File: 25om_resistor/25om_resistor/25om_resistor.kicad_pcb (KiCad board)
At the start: 2 copper layers, 24.2 x 21.9 mm, 11 parts, among them J1 Conn_01x02_Female

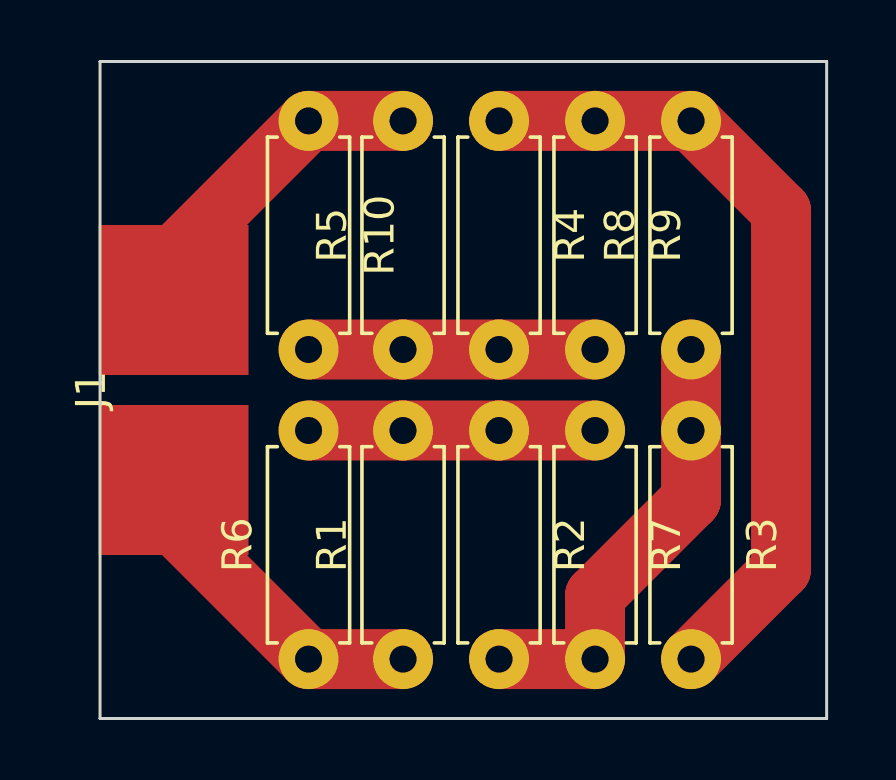
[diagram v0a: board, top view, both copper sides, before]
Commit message: Cleanup
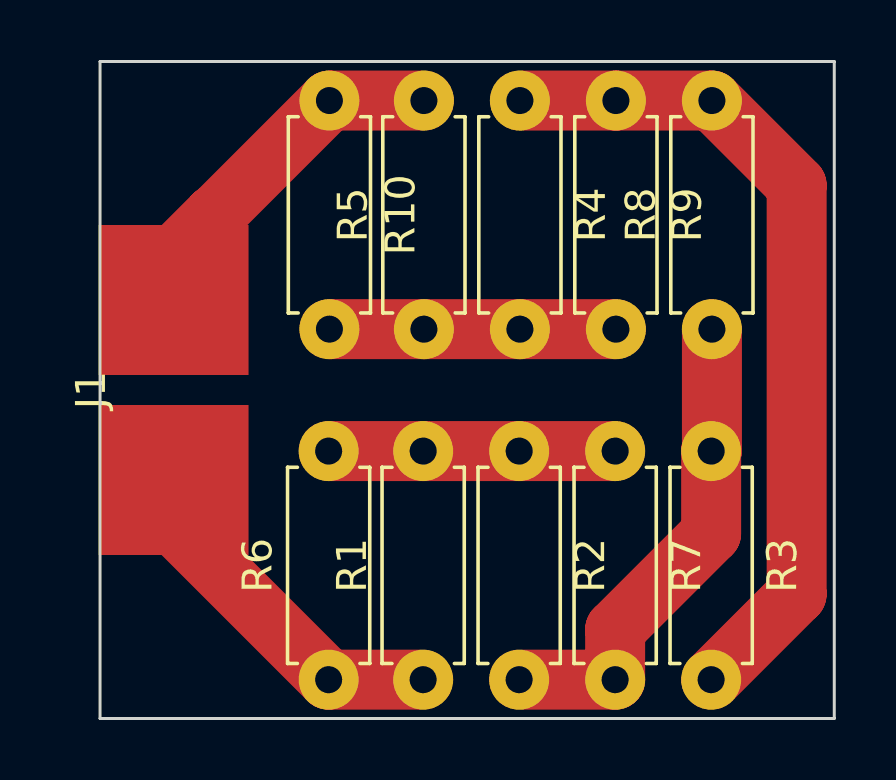
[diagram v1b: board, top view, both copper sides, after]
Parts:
- moved R4 0.97 mm to (64.8, 28.7)
- moved R9 0.97 mm to (68.0, 28.7)
- moved R10 0.97 mm to (58.4, 28.7)
- moved R5 0.97 mm to (61.6, 36.3)
- moved R8 0.97 mm to (71.2, 36.3)
- moved R1 0.96 mm to (61.6, 48.0)
- moved R2 0.96 mm to (64.8, 40.4)
- moved R3 0.96 mm to (71.2, 40.4)
- moved R6 0.96 mm to (58.4, 48.0)
- moved R7 0.96 mm to (68.0, 40.4)
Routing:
- net Net-(R2-Pad2): track 14.8 -> 16.2 mm
- net Net-(R3-Pad2): track 26.8 -> 28.1 mm
- net Net-(J1-Pad2): track 11.0 -> 12.0 mm
- net Net-(J1-Pad1): track 11.0 -> 11.9 mm
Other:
- board size 24.2 x 21.9 mm -> 24.5 x 21.9 mm
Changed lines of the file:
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@@
     (pad_to_mask_clearance 0)
     (pcbplotparams
-      (layerselection 0x00010fc_ffffffff)
+      (layerselection 0x0001000_7fffffff)
       (disableapertmacros false)
       (usegerberextensions false)
@@
       (outputformat 1)
       (mirror false)
-      (drillshape 1)
+      (drillshape 0)
       (scaleselection 1)
-      (outputdirectory "")
+      (outputdirectory "out/")
     )
   )
@@
   (net 6 "Net-(R10-Pad2)")
   (footprint "Resistor_THT:R_Axial_DIN0207_L6.3mm_D2.5mm_P7.62mm_Horizontal" (layer "F.Cu")
-    (at 67.3 39.7 -90)
+    (at 67.97 40.386 -90)
     (descr "Resistor, Axial_DIN0207 series, Axial, Horizontal, pin pitch=7.62mm, 0.25W = 1/4W, length*diameter=6.3*2.5mm^2, http://cdn-reichelt.de/documents/datenblatt/B400/1_4W%23YAG.pdf")
     (tags "Resistor Axial_DIN0207 series Axial Horizontal pin pitch 7.62mm 0.25W = 1/4W length 6.3mm diameter 2.5mm")
@@
   )
   (footprint "Resistor_THT:R_Axial_DIN0207_L6.3mm_D2.5mm_P7.62mm_Horizontal" (layer "F.Cu")
-    (at 57.75 47.32 90)
+    (at 58.42 48.006 90)
     (descr "Resistor, Axial_DIN0207 series, Axial, Horizontal, pin pitch=7.62mm, 0.25W = 1/4W, length*diameter=6.3*2.5mm^2, http://cdn-reichelt.de/documents/datenblatt/B400/1_4W%23YAG.pdf")
     (tags "Resistor Axial_DIN0207 series Axial Horizontal pin pitch 7.62mm 0.25W = 1/4W length 6.3mm diameter 2.5mm")
@@
   )
   (footprint "Resistor_THT:R_Axial_DIN0207_L6.3mm_D2.5mm_P7.62mm_Horizontal" (layer "F.Cu")
-    (at 70.5 37 90)
+    (at 71.195 36.322 90)
     (descr "Resistor, Axial_DIN0207 series, Axial, Horizontal, pin pitch=7.62mm, 0.25W = 1/4W, length*diameter=6.3*2.5mm^2, http://cdn-reichelt.de/documents/datenblatt/B400/1_4W%23YAG.pdf")
     (tags "Resistor Axial_DIN0207 series Axial Horizontal pin pitch 7.62mm 0.25W = 1/4W length 6.3mm diameter 2.5mm")
@@
   )
   (footprint "Resistor_THT:R_Axial_DIN0207_L6.3mm_D2.5mm_P7.62mm_Horizontal" (layer "F.Cu")
-    (at 60.9 37 90)
+    (at 61.595 36.322 90)
     (descr "Resistor, Axial_DIN0207 series, Axial, Horizontal, pin pitch=7.62mm, 0.25W = 1/4W, length*diameter=6.3*2.5mm^2, http://cdn-reichelt.de/documents/datenblatt/B400/1_4W%23YAG.pdf")
     (tags "Resistor Axial_DIN0207 series Axial Horizontal pin pitch 7.62mm 0.25W = 1/4W length 6.3mm diameter 2.5mm")
@@
   )
   (footprint "Resistor_THT:R_Axial_DIN0207_L6.3mm_D2.5mm_P7.62mm_Horizontal" (layer "F.Cu")
-    (at 64.1 29.38 -90)
+    (at 64.795 28.702 -90)
     (descr "Resistor, Axial_DIN0207 series, Axial, Horizontal, pin pitch=7.62mm, 0.25W = 1/4W, length*diameter=6.3*2.5mm^2, http://cdn-reichelt.de/documents/datenblatt/B400/1_4W%23YAG.pdf")
     (tags "Resistor Axial_DIN0207 series Axial Horizontal pin pitch 7.62mm 0.25W = 1/4W length 6.3mm diameter 2.5mm")
@@
   )
   (footprint "Resistor_THT:R_Axial_DIN0207_L6.3mm_D2.5mm_P7.62mm_Horizontal" (layer "F.Cu")
-    (at 70.5 39.7 -90)
+    (at 71.17 40.386 -90)
     (descr "Resistor, Axial_DIN0207 series, Axial, Horizontal, pin pitch=7.62mm, 0.25W = 1/4W, length*diameter=6.3*2.5mm^2, http://cdn-reichelt.de/documents/datenblatt/B400/1_4W%23YAG.pdf")
     (tags "Resistor Axial_DIN0207 series Axial Horizontal pin pitch 7.62mm 0.25W = 1/4W length 6.3mm diameter 2.5mm")
@@
   )
   (footprint "Resistor_THT:R_Axial_DIN0207_L6.3mm_D2.5mm_P7.62mm_Horizontal" (layer "F.Cu")
-    (at 57.75 29.38 -90)
+    (at 58.445 28.702 -90)
     (descr "Resistor, Axial_DIN0207 series, Axial, Horizontal, pin pitch=7.62mm, 0.25W = 1/4W, length*diameter=6.3*2.5mm^2, http://cdn-reichelt.de/documents/datenblatt/B400/1_4W%23YAG.pdf")
     (tags "Resistor Axial_DIN0207 series Axial Horizontal pin pitch 7.62mm 0.25W = 1/4W length 6.3mm diameter 2.5mm")
@@
   )
   (footprint "Resistor_THT:R_Axial_DIN0207_L6.3mm_D2.5mm_P7.62mm_Horizontal" (layer "F.Cu")
-    (at 60.9 47.32 90)
+    (at 61.57 48.006 90)
     (descr "Resistor, Axial_DIN0207 series, Axial, Horizontal, pin pitch=7.62mm, 0.25W = 1/4W, length*diameter=6.3*2.5mm^2, http://cdn-reichelt.de/documents/datenblatt/B400/1_4W%23YAG.pdf")
     (tags "Resistor Axial_DIN0207 series Axial Horizontal pin pitch 7.62mm 0.25W = 1/4W length 6.3mm diameter 2.5mm")
@@
   )
   (footprint "Resistor_THT:R_Axial_DIN0207_L6.3mm_D2.5mm_P7.62mm_Horizontal" (layer "F.Cu")
-    (at 64.1 39.7 -90)
+    (at 64.77 40.386 -90)
     (descr "Resistor, Axial_DIN0207 series, Axial, Horizontal, pin pitch=7.62mm, 0.25W = 1/4W, length*diameter=6.3*2.5mm^2, http://cdn-reichelt.de/documents/datenblatt/B400/1_4W%23YAG.pdf")
     (tags "Resistor Axial_DIN0207 series Axial Horizontal pin pitch 7.62mm 0.25W = 1/4W length 6.3mm diameter 2.5mm")
@@
       (effects (font (size 1 1) (thickness 0.15)))
     )
-    (fp_text value "Conn_01x02_Female" (at 3 2.75 90) (layer "F.Fab")
+    (fp_text value "Conn_01x02_Female" (at 2.992 4.115 90) (layer "F.Fab")
       (effects (font (size 1 1) (thickness 0.15)))
     )
@@
   )
   (footprint "Resistor_THT:R_Axial_DIN0207_L6.3mm_D2.5mm_P7.62mm_Horizontal" (layer "F.Cu")
-    (at 67.3 29.38 -90)
+    (at 67.995 28.702 -90)
     (descr "Resistor, Axial_DIN0207 series, Axial, Horizontal, pin pitch=7.62mm, 0.25W = 1/4W, length*diameter=6.3*2.5mm^2, http://cdn-reichelt.de/documents/datenblatt/B400/1_4W%23YAG.pdf")
     (tags "Resistor Axial_DIN0207 series Axial Horizontal pin pitch 7.62mm 0.25W = 1/4W length 6.3mm diameter 2.5mm")
@@
     )
   )
-  (gr_rect (start 50.8 27.4) (end 75.02 49.3) (layer "Edge.Cuts") (width 0.1) (fill none))
-  (segment (start 57.75 47.32) (end 60.9 47.32) (width 2) (layer "F.Cu") (net 1))
-  (segment (start 53.25 42.82) (end 57.75 47.32) (width 2) (layer "F.Cu") (net 1))
-  (segment (start 53.25 41.35) (end 53.25 42.82) (width 2) (layer "F.Cu") (net 1))
-  (segment (start 53.25 33.88) (end 57.75 29.38) (width 2) (layer "F.Cu") (net 2))
-  (segment (start 53.25 35.35) (end 53.25 33.88) (width 2) (layer "F.Cu") (net 2))
-  (segment (start 57.75 29.38) (end 60.9 29.38) (width 2) (layer "F.Cu") (net 2))
-  (segment (start 57.75 39.7) (end 60.9 39.7) (width 2) (layer "F.Cu") (net 3))
-  (segment (start 60.9 39.7) (end 64.1 39.7) (width 2) (layer "F.Cu") (net 3))
-  (segment (start 64.1 39.7) (end 67.3 39.7) (width 2) (layer "F.Cu") (net 3))
-  (segment (start 64.1 47.32) (end 67.3 47.32) (width 2) (layer "F.Cu") (net 4))
-  (segment (start 67.3 47.32) (end 67.3 45.2) (width 2) (layer "F.Cu") (net 4))
-  (segment (start 67.3 45.2) (end 70.5 42) (width 2) (layer "F.Cu") (net 4))
-  (segment (start 70.5 42) (end 70.5 39.7) (width 2) (layer "F.Cu") (net 4))
-  (segment (start 70.5 39.7) (end 70.5 37) (width 2) (layer "F.Cu") (net 4))
-  (segment (start 73.5 32.38) (end 73.5 44.32) (width 2) (layer "F.Cu") (net 5))
-  (segment (start 73.5 44.32) (end 70.5 47.32) (width 2) (layer "F.Cu") (net 5))
-  (segment (start 67.3 29.38) (end 70.5 29.38) (width 2) (layer "F.Cu") (net 5))
-  (segment (start 64.1 29.38) (end 67.3 29.38) (width 2) (layer "F.Cu") (net 5))
-  (segment (start 70.5 29.38) (end 73.5 32.38) (width 2) (layer "F.Cu") (net 5))
-  (segment (start 64.1 37) (end 67.3 37) (width 2) (layer "F.Cu") (net 6))
-  (segment (start 64.1 37) (end 60.9 37) (width 2) (layer "F.Cu") (net 6))
-  (segment (start 57.75 37) (end 60.9 37) (width 2) (layer "F.Cu") (net 6))
+  (gr_rect (start 50.8 27.4) (end 75.274 49.3) (layer "Edge.Cuts") (width 0.1) (fill none))
+  (segment (start 58.42 48.006) (end 61.57 48.006) (width 2) (layer "F.Cu") (net 1))
+  (segment (start 53.25 41.35) (end 53.25 42.836) (width 2) (layer "F.Cu") (net 1))
+  (segment (start 53.25 42.836) (end 58.42 48.006) (width 2) (layer "F.Cu") (net 1))
+  (segment (start 54.635 32.512) (end 54.61 32.512) (width 2) (layer "F.Cu") (net 2))
+  (segment (start 54.61 32.512) (end 53.25 33.872) (width 2) (layer "F.Cu") (net 2))
+  (segment (start 53.25 33.872) (end 53.25 35.35) (width 2) (layer "F.Cu") (net 2))
+  (segment (start 58.445 28.702) (end 54.635 32.512) (width 2) (layer "F.Cu") (net 2))
+  (segment (start 58.445 28.702) (end 61.595 28.702) (width 2) (layer "F.Cu") (net 2))
+  (segment (start 58.42 40.386) (end 61.57 40.386) (width 2) (layer "F.Cu") (net 3))
+  (segment (start 61.57 40.386) (end 64.77 40.386) (width 2) (layer "F.Cu") (net 3))
+  (segment (start 64.77 40.386) (end 67.97 40.386) (width 2) (layer "F.Cu") (net 3))
+  (segment (start 64.77 48.006) (end 67.97 48.006) (width 2) (layer "F.Cu") (net 4))
+  (segment (start 71.195 36.322) (end 71.195 40.361) (width 2) (layer "F.Cu") (net 4))
+  (segment (start 67.97 48.006) (end 67.97 46.33) (width 2) (layer "F.Cu") (net 4))
+  (segment (start 71.195 40.361) (end 71.17 40.386) (width 2) (layer "F.Cu") (net 4))
+  (segment (start 71.17 43.13) (end 71.17 40.386) (width 2) (layer "F.Cu") (net 4))
+  (segment (start 67.97 46.33) (end 71.17 43.13) (width 2) (layer "F.Cu") (net 4))
+  (segment (start 67.995 28.702) (end 71.195 28.702) (width 2) (layer "F.Cu") (net 5))
+  (segment (start 74.02 31.527) (end 71.195 28.702) (width 2) (layer "F.Cu") (net 5))
+  (segment (start 64.795 28.702) (end 67.995 28.702) (width 2) (layer "F.Cu") (net 5))
+  (segment (start 74.02 45.156) (end 74.02 31.527) (width 2) (layer "F.Cu") (net 5))
+  (segment (start 71.17 48.006) (end 74.02 45.156) (width 2) (layer "F.Cu") (net 5))
+  (segment (start 64.795 36.322) (end 67.995 36.322) (width 2) (layer "F.Cu") (net 6))
+  (segment (start 64.795 36.322) (end 61.595 36.322) (width 2) (layer "F.Cu") (net 6))
+  (segment (start 58.445 36.322) (end 61.595 36.322) (width 2) (layer "F.Cu") (net 6))
 )
